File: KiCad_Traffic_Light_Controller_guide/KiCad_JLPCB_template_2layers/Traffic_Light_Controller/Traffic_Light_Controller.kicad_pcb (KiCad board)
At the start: 2 copper layers, 124.2 x 91.4 mm, 65 parts, among them J1 Conn_02x08_Odd_Even, J2 Conn_02x08_Odd_Even, J3 Conn_02x05_Odd_Even, J4 +5V, SW1 RST, SW2 OVRRIDE, SW3 EN, U1 SM420561N, U2 SM420561N, U3 LM1117DT-3.3

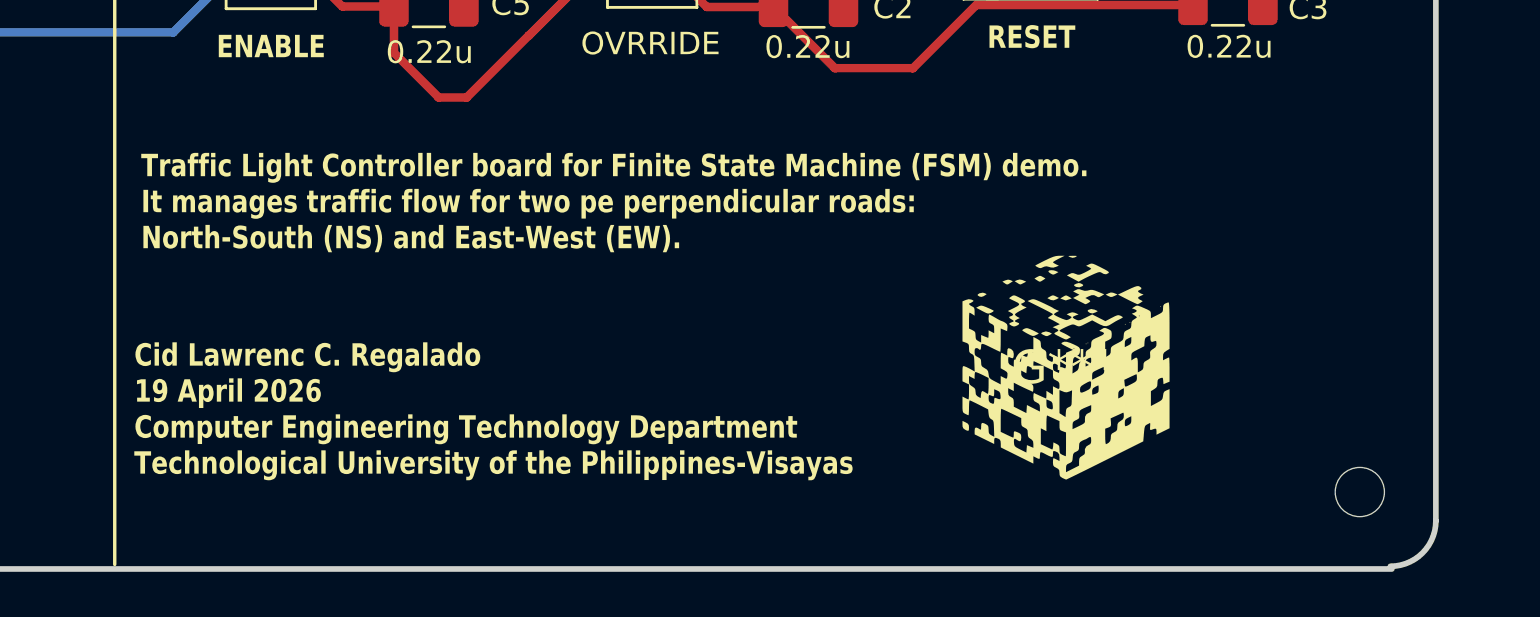
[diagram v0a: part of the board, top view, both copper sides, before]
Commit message: n
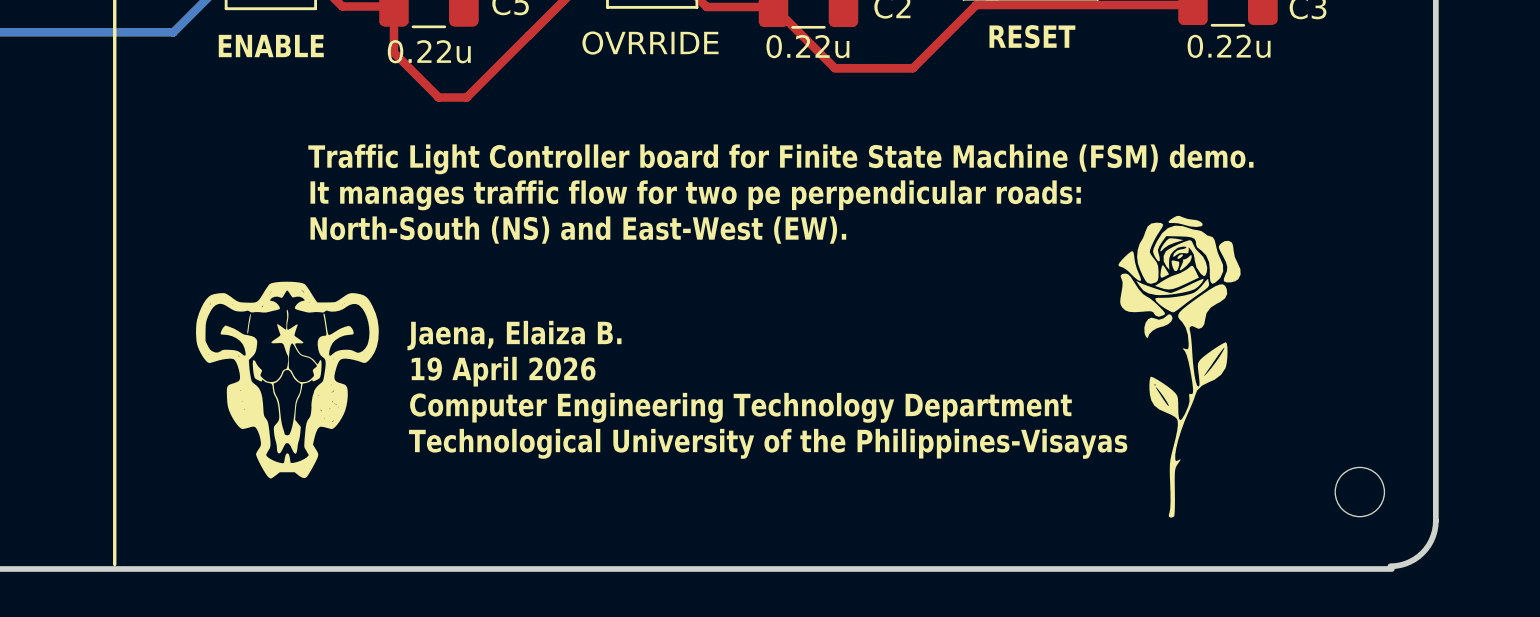
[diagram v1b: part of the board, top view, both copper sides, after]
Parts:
- removed the G*** at (182.8, 135.6)
- added G***: LOGO, LOGO, F.Cu at (188.0, 135.5)
- added G***: LOGO, LOGO, F.Cu at (148.0, 136.5)
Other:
- board text added: "Jaena, Elaiza B. 19 April 2026 Computer Engineering Technology Department Technological University of the Philippines-Visayas"
- board text removed: "Cid Lawrenc C. Regalado 19 April 2026 Computer Engineering Technology Department Technological University of the Philippines-Visayas"
